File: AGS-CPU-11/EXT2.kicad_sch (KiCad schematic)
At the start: 14 parts, among them P3 EXT2, Q11 2SD1819A

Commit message: Release: AGB-CPU-11 rev D
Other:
- title: AGS-CPU-11 - EXT2 port -> AGS-CPU-11
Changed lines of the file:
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@@
   (paper "A4")
   (title_block
-    (title "AGS-CPU-11 - EXT2 port")
-    (date "2021-07-26")
-    (rev "C")
+    (title "AGS-CPU-11")
+    (date "2022-01-02")
+    (rev "D")
     (company "https://gekkio.fi")
     (comment 1 "https://github.com/Gekkio/gb-schematics")

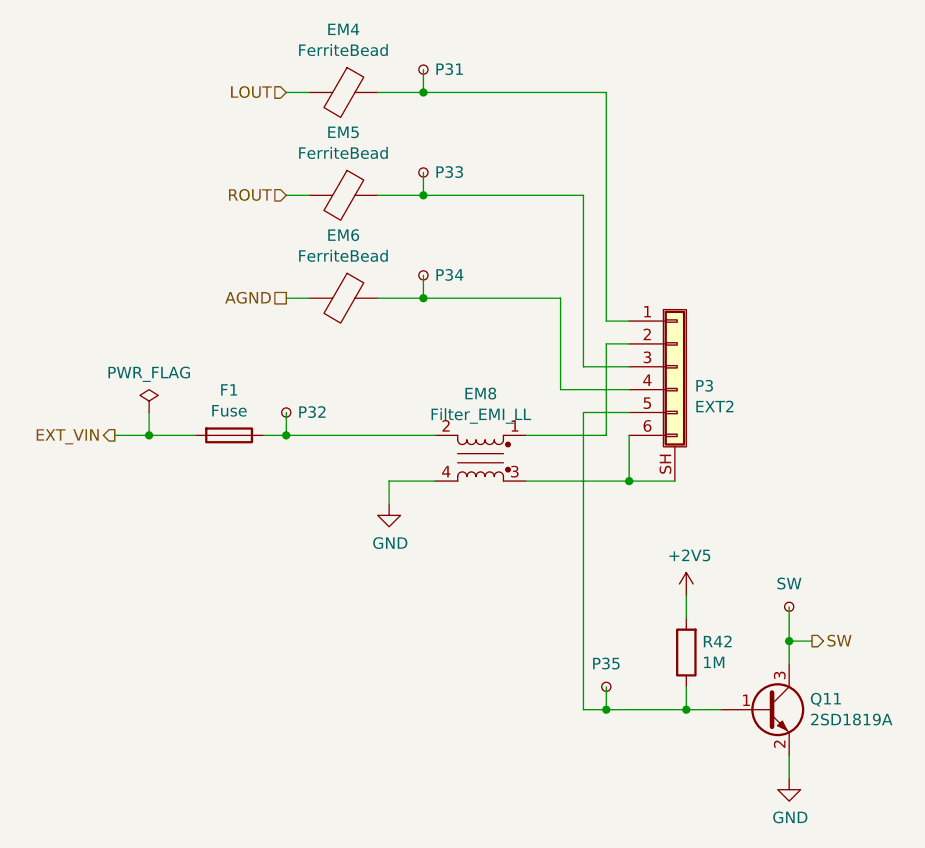
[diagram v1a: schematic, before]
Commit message: Update to latest KiCad
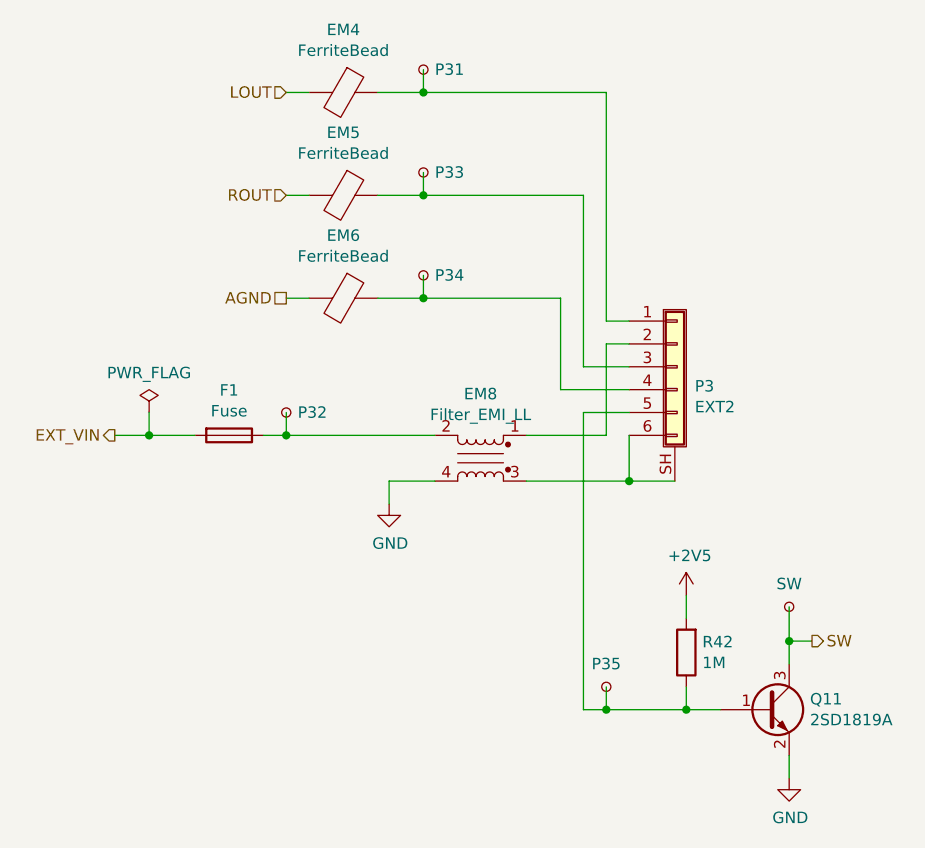
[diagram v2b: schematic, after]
